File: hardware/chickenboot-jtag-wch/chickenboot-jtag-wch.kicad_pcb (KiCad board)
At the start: 2 copper layers, 28.2 x 18 mm, 28 parts, among them CN1 69168-106HLF, J1 USB_C_Receptacle_USB2.0, J2 Conn_01x03, J4 Conn_01x03, Q1 WPM2093-3/TR, SW1 SW_Push, U1 CH32X035F8U6, U2 HT7533-1, U3 USBLC6-2P6, U4 IS25WP016D-JULE-TR

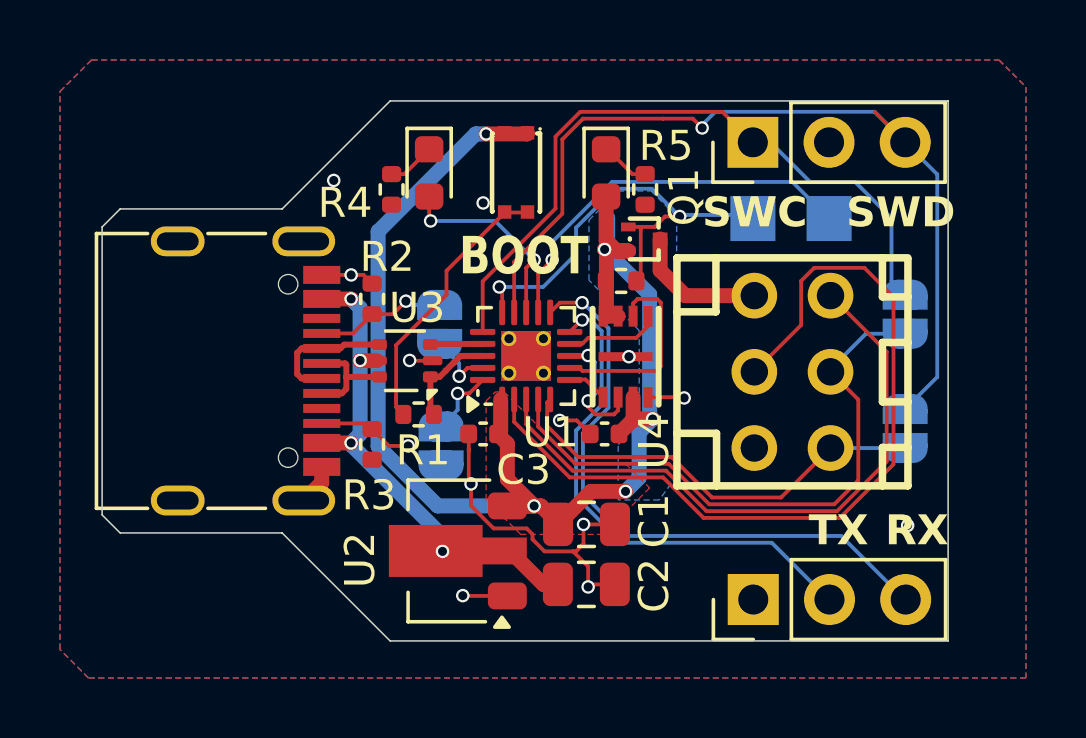
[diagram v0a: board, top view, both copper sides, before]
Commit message: fix vias and tracks to pass DFM
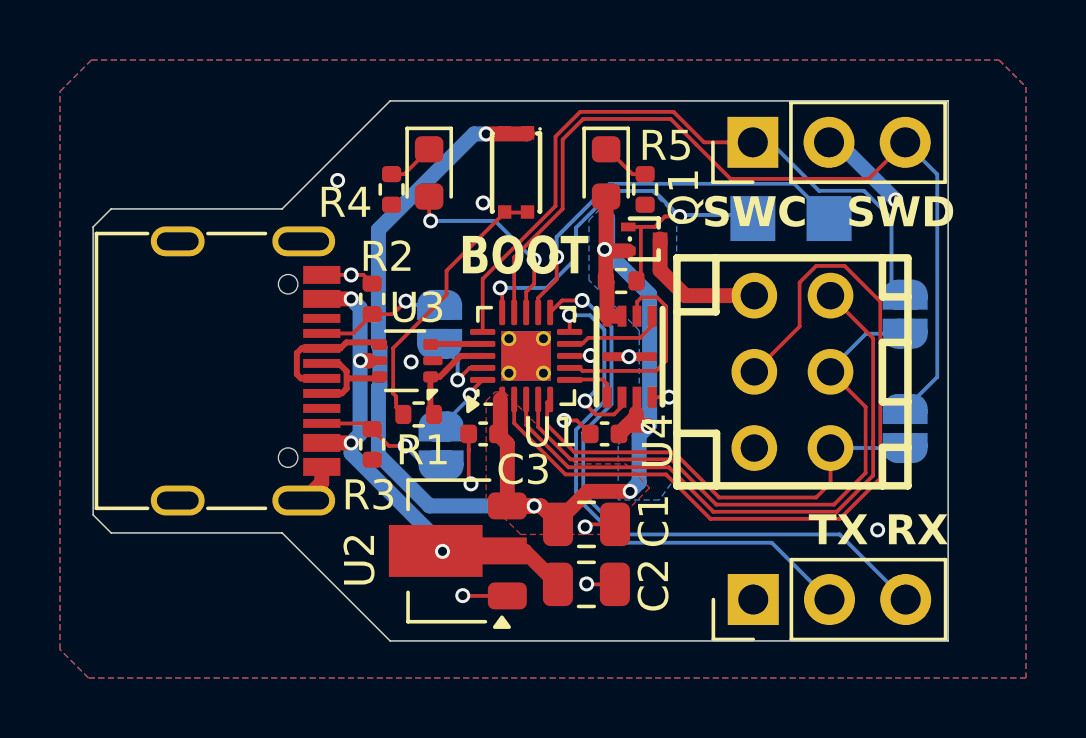
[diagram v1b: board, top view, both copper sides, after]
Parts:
- moved U4 0.13 mm to (92.8, 114.6)
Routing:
- net GND: track 18.9 -> 13.5 mm, vias 12 -> 13
- net /SWDIO: track 30.2 -> 29.2 mm, vias 1 -> 0
- net +3V3: track 47.2 -> 46.5 mm
- net JTAG_TDO: track 14.6 -> 15.3 mm
- net /TX: track 17.1 -> 17.7 mm
- net JTAG_TDI: track 28.4 -> 27.8 mm
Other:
- board size 28.2 x 18 mm -> 28.5 x 18 mm
